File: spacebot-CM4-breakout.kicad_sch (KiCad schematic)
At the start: 2 parts, among them J1 Conn_02x12_Counter_Clockwise, U1 Compute_Module_4_Connectors

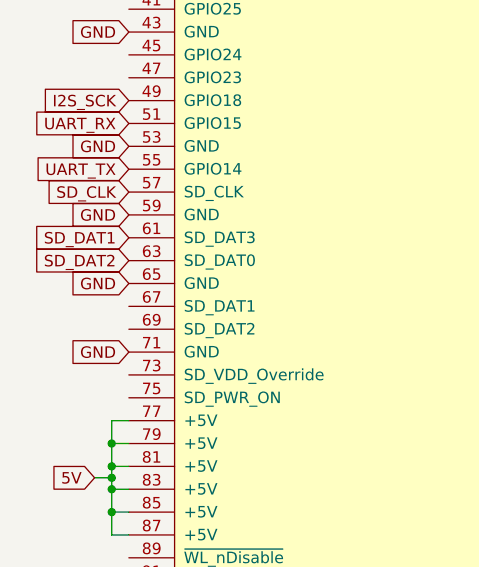
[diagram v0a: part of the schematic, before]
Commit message: updates
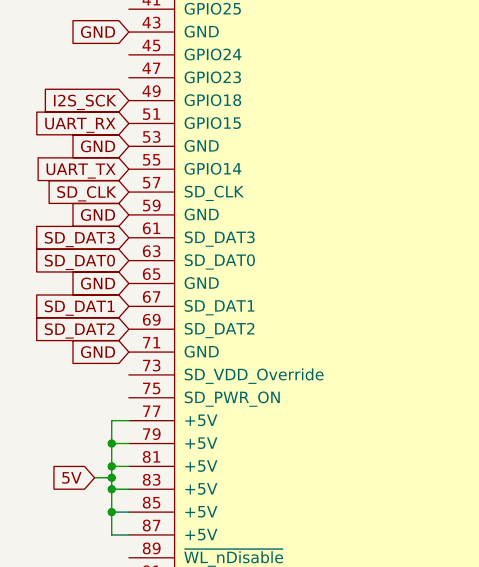
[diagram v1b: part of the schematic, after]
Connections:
- net SD_DAT0: now also U1.63 (SD_DAT0)
- net SD_DAT1: now also U1.67 (SD_DAT1); no longer U1.61 (SD_DAT3)
- net SD_DAT2: now also U1.69 (SD_DAT2); no longer U1.63 (SD_DAT0)
- net SD_DAT3: now also U1.61 (SD_DAT3)
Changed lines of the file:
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@@
+    )
+  )
+  (global_label "SD_DAT1" (shape input) (at 53.34 113.03 180) (fields_autoplaced)
+    (effects (font (size 1.27 1.27)) (justify right))
+    (property "Intersheet References" "${INTERSHEET_REFS}" (id 0) (at 42.944 112.9506 0)
+      (effects (font (size 1.27 1.27)) (justify right) hide)
     )
   )
@@
     )
   )
-  (global_label "SD_DAT1" (shape input) (at 53.34 105.41 180) (fields_autoplaced)
+  (global_label "SD_DAT3" (shape input) (at 53.34 105.41 180) (fields_autoplaced)
     (effects (font (size 1.27 1.27)) (justify right))
     (property "Intersheet References" "${INTERSHEET_REFS}" (id 0) (at 42.944 105.3306 0)
@@
     )
   )
-  (global_label "SD_DAT2" (shape input) (at 53.34 107.95 180) (fields_autoplaced)
+  (global_label "SD_DAT0" (shape input) (at 53.34 107.95 180) (fields_autoplaced)
     (effects (font (size 1.27 1.27)) (justify right))
     (property "Intersheet References" "${INTERSHEET_REFS}" (id 0) (at 42.944 107.8706 0)
@@
     )
   )
+  (global_label "SD_DAT2" (shape input) (at 53.34 115.57 180) (fields_autoplaced)
+    (effects (font (size 1.27 1.27)) (justify right))
+    (property "Intersheet References" "${INTERSHEET_REFS}" (id 0) (at 42.944 115.4906 0)
+      (effects (font (size 1.27 1.27)) (justify right) hide)
+    )
+  )

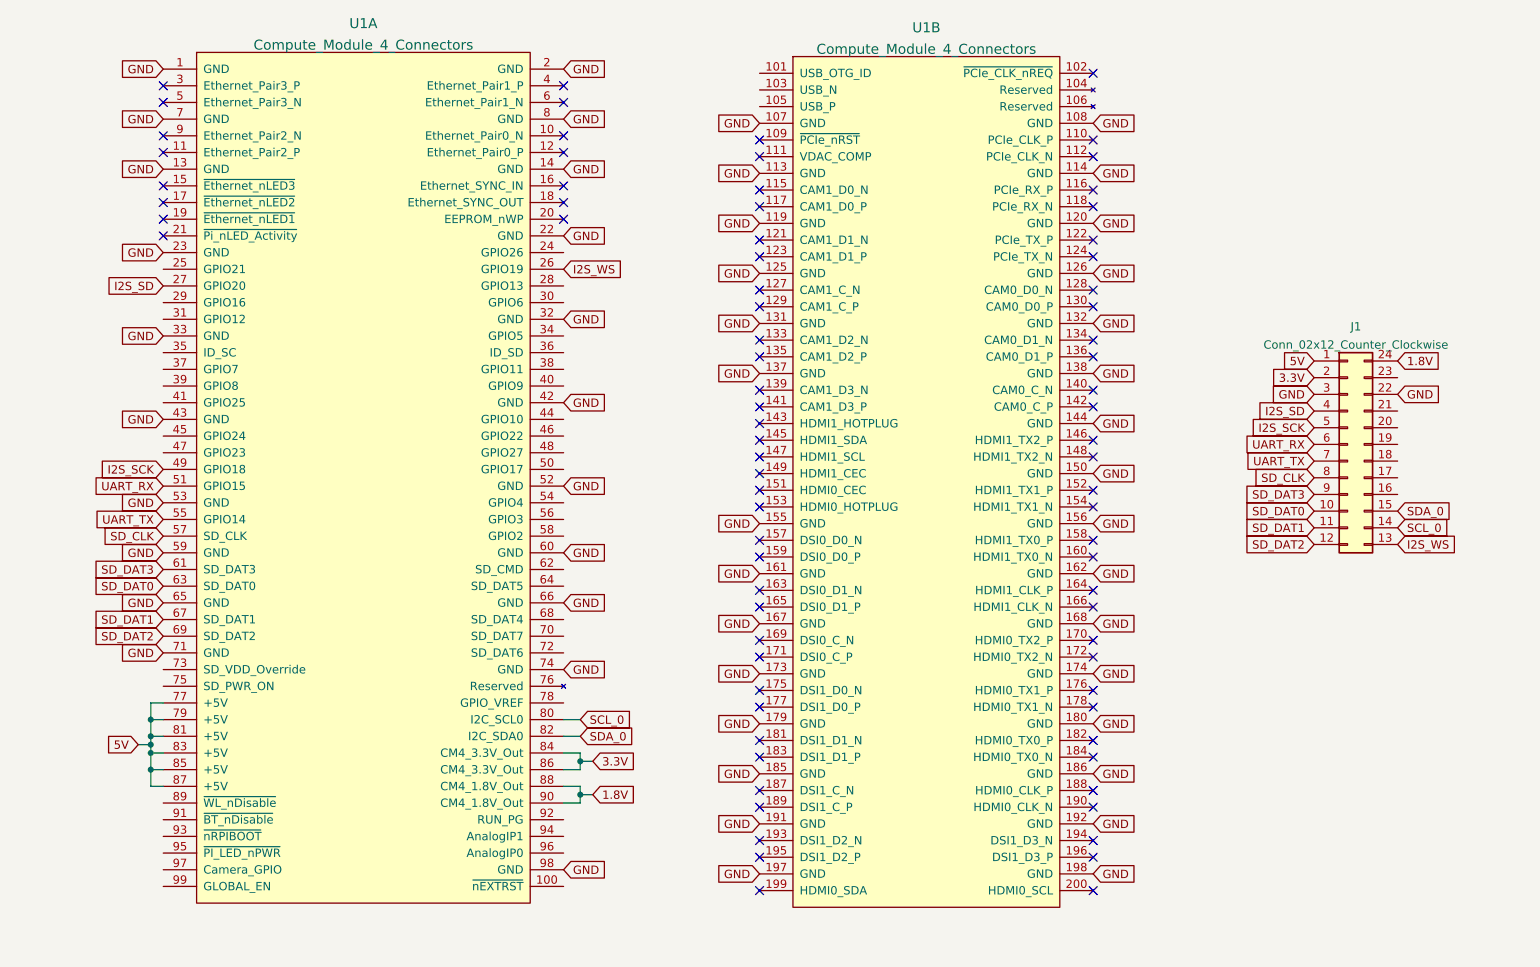
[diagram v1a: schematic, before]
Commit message: updates
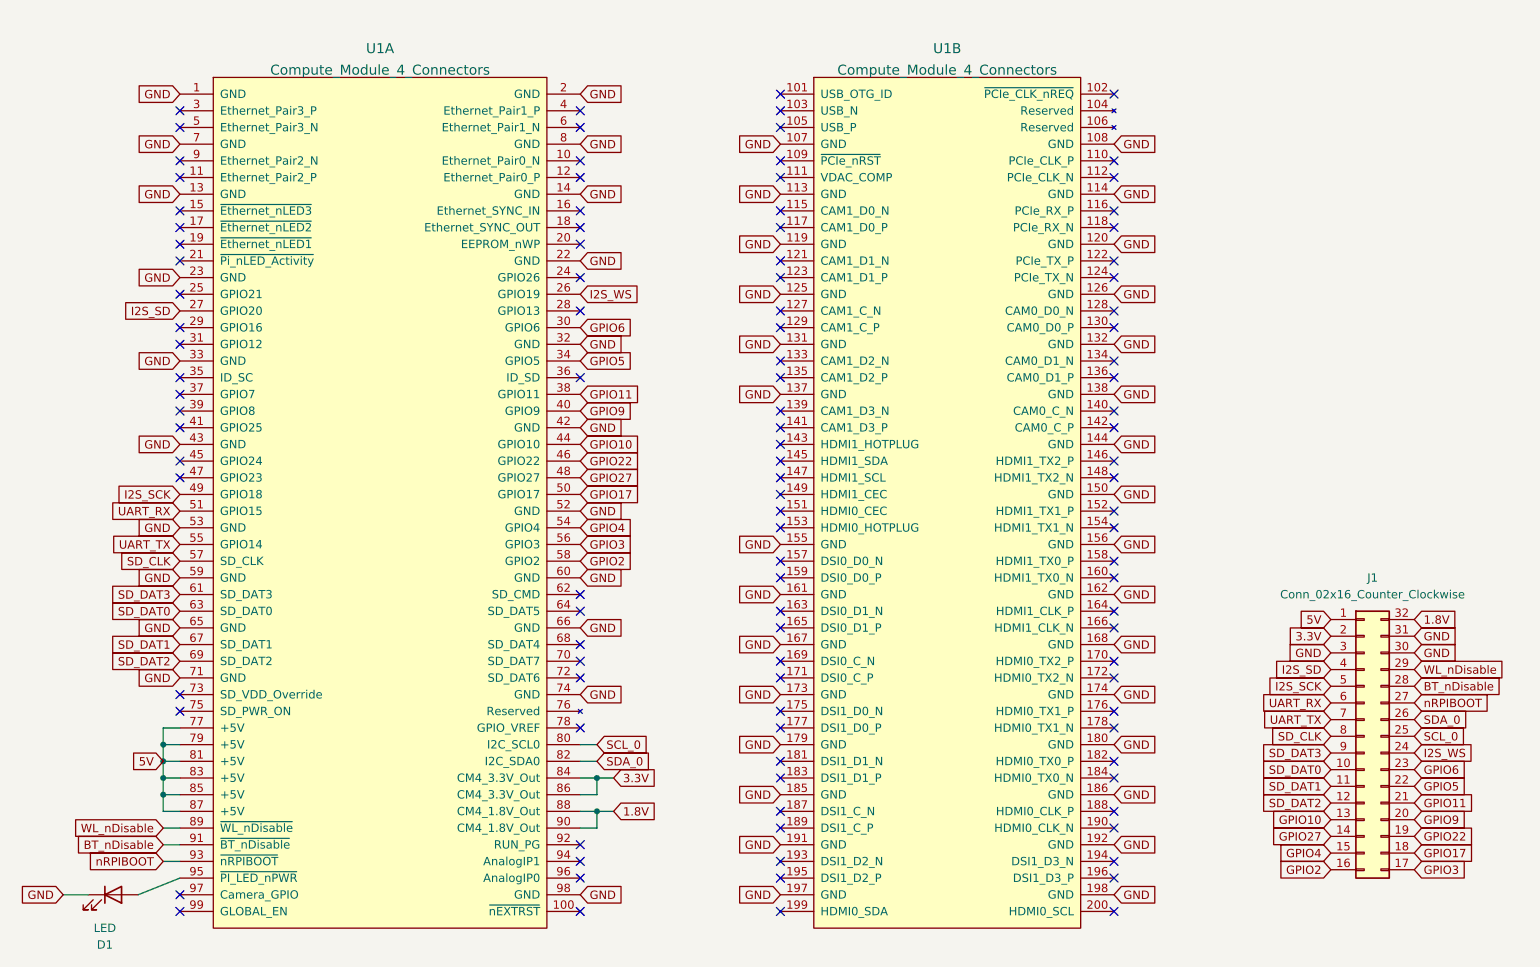
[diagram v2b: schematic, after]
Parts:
- removed J1: Conn_02x12_Counter_Clockwise, Connector_PinHeader_2.54mm:PinHeader_2x12_P2.54mm_Horizontal, symbol Connector_Generic:Conn_02x12_Counter_Clockwise
- added D1: LED, LED_THT:LED_D3.0mm, symbol Device:LED
- added J1: Conn_02x16_Counter_Clockwise, Connector_PinHeader_2.54mm:PinHeader_2x16_P2.54mm_Horizontal, symbol Connector_Generic:Conn_02x16_Counter_Clockwise
- U1: footprint (none) -> CM4:Raspberry-Pi-4-Compute-Module
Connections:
- net 1.8V: now also J1.32 (Pin_32)
- net 3.3V: now also J1.2 (Pin_2)
- net 5V: now also J1.1 (Pin_1)
- net GND: now also D1.1 (K), J1.3 (Pin_3), J1.30 (Pin_30), J1.31 (Pin_31)
- net I2S_SCK: now also J1.5 (Pin_5)
- net I2S_SD: now also J1.4 (Pin_4)
- net I2S_WS: now also J1.24 (Pin_24)
- net SCL_0: now also J1.25 (Pin_25)
- net SDA_0: now also J1.26 (Pin_26)
- net SD_CLK: now also J1.8 (Pin_8)
- net SD_DAT0: now also J1.10 (Pin_10)
- net SD_DAT1: now also J1.11 (Pin_11)
- net SD_DAT2: now also J1.12 (Pin_12)
- net SD_DAT3: now also J1.9 (Pin_9)
- net UART_RX: now also J1.6 (Pin_6)
- net UART_TX: now also J1.7 (Pin_7)
- net GPIO6: now reaches U1.30 (GPIO6)
- net GPIO6: now also J1.23 (Pin_23)
- net GPIO5: now reaches U1.34 (GPIO5)
- net GPIO5: now also J1.22 (Pin_22)
- net GPIO11: now reaches U1.38 (GPIO11)
- net GPIO11: now also J1.21 (Pin_21)
- net GPIO9: now reaches U1.40 (GPIO9)
- net GPIO9: now also J1.20 (Pin_20)
- net GPIO10: now reaches U1.44 (GPIO10)
- net GPIO10: now also J1.13 (Pin_13)
- net GPIO22: now reaches U1.46 (GPIO22)
- net GPIO22: now also J1.19 (Pin_19)
- net GPIO27: now reaches U1.48 (GPIO27)
- net GPIO27: now also J1.14 (Pin_14)
- net GPIO17: now reaches U1.50 (GPIO17)
- net GPIO17: now also J1.18 (Pin_18)
- net GPIO4: now reaches U1.54 (GPIO4)
- net GPIO4: now also J1.15 (Pin_15)
- net GPIO3: now reaches U1.56 (GPIO3)
- net GPIO3: now also J1.17 (Pin_17)
- net GPIO2: now reaches U1.58 (GPIO2)
- net GPIO2: now also J1.16 (Pin_16)
- net WL_nDisable: now reaches U1.89 (~{WL_nDisable})
- net WL_nDisable: now also J1.29 (Pin_29)
- net BT_nDisable: now reaches U1.91 (~{BT_nDisable})
- net BT_nDisable: now also J1.28 (Pin_28)
- net nRPIBOOT: now reaches U1.93 (~{nRPIBOOT})
- net nRPIBOOT: now also J1.27 (Pin_27)
- net at U1.95 (~{PI_LED_nPWR}): now also D1.2 (A)
- no-connect marks 80 -> 109
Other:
- moved on the sheet: U1A, U1B
